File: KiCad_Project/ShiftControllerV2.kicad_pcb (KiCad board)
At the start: 2 copper layers, 102.9 x 43.2 mm, 25 parts, among them J1 SOLENOID, J2 PWR + I/O, Q1 BTN8982TA, Q2 BTN8982TA, U1 ControllerBoardV1

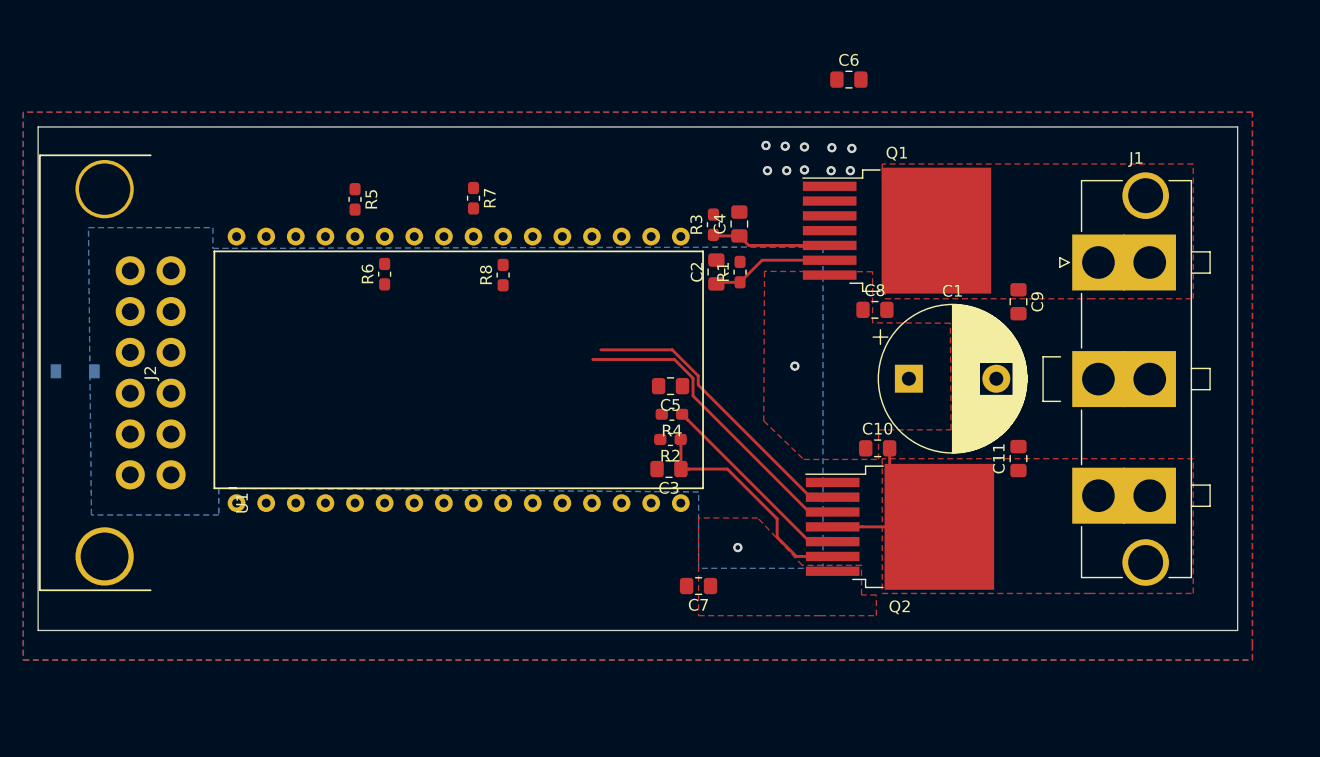
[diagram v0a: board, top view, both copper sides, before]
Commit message: Layout almost complete
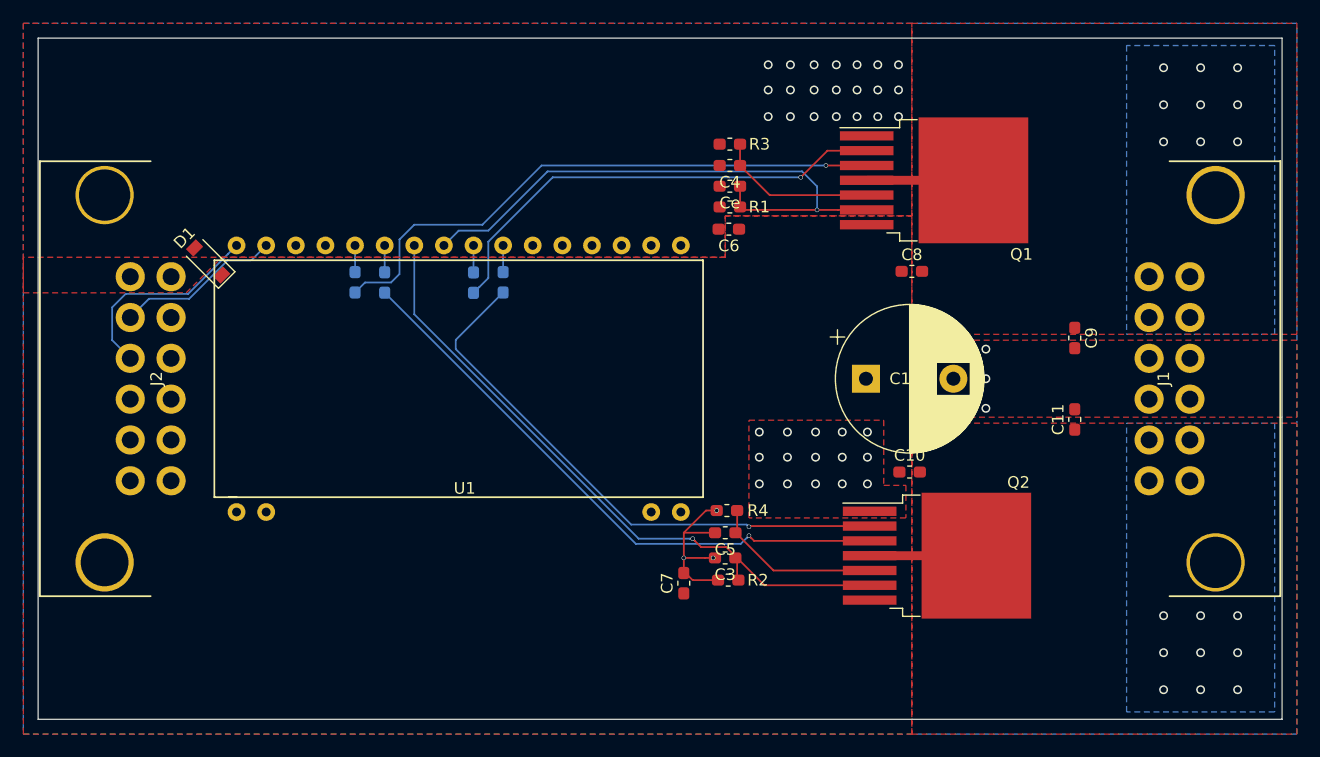
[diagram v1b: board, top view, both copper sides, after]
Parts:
- removed C2: 1n, Capacitor_SMD:C_0805_2012Metric_Pad1.15x1.40mm_HandSolder
- added Ce: 1n, Capacitor_SMD:C_0603_1608Metric_Pad1.05x0.95mm_HandSolder, F.Cu at (135.5, 81.3)
- C10, C11, C3, C4, C5, C6, C7, C8, C9: footprint Capacitor_SMD:C_0805_2012Metric_Pad1.15x1.40mm_HandSolder -> Capacitor_SMD:C_0603_1608Metric_Pad1.05x0.95mm_HandSolder
- D1: moved to F.Cu
- J1: value SOLENOID -> Conn_02x06_Top_Bottom; footprint Connector_Molex:Molex_Mini-Fit_Sr_42819-32XX_1x03_P10.00mm_Vertical -> Lukas_Library:MX120G
- J2: value PWR + I/O -> Conn_02x06_Top_Bottom
- R5, R6, R7, R8: moved to B.Cu
- moved C6 16.4 mm to (135.4, 85.0), turned to 180 degrees
- moved D1 14.8 mm to (90.8, 87.7), turned to 135 degrees
- moved C5 13.4 mm to (135.1, 111.0)
- moved R2 13.0 mm to (135.4, 115.1)
- moved J1 11.7 mm to (173.2, 97.8), turned to 270 degrees
- moved R4 9.51 mm to (135.3, 109.1)
- moved C3 9.01 mm to (135.1, 113.2)
- moved R7 7.24 mm to (113.5, 89.5), turned to 90 degrees
- moved R5 7.11 mm to (103.4, 89.5), turned to 90 degrees
- moved R3 7.05 mm to (135.5, 77.7), turned to 180 degrees
- moved C11 5.88 mm to (165.1, 101.3)
- moved C9 5.74 mm to (165.1, 94.3)
- moved R1 5.66 mm to (135.5, 83.1), turned to 180 degrees
- moved Q1 5.36 mm to (153.0, 80.8)
- moved C4 5.08 mm to (135.5, 79.5), turned to 180 degrees
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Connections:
- J1 pad 1: OUT1 -> OUT2
- J1 pad 2: GND -> OUT2
- J1 pad 3: OUT2 -> GND
- J2 pad 1: +12V -> GND
- J2 pad 11: GND -> (no net)
- J2 pad 12: +12V -> GND
- J2 pad 2: GND -> +12V
- J2 pad 3: CANL -> +12V
- J2 pad 4: CANH -> +12V
- J2 pad 5: GND -> +12V
- J2 pad 6: +12V -> GND
- J2 pad 7: +12V -> GND
- J2 pad 8: GND -> CANH
- J2 pad 9: (no net) -> CANL
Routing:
- net INH1: track 1.90 -> 50.1 mm, vias 0 -> 1
- net CURRENT1: track 10.6 -> 49.9 mm, vias 0 -> 1
- net IN1: track 1.90 -> 40.6 mm, vias 0 -> 1
- net CURRENT2: track 19.6 -> 56.5 mm, vias 0 -> 1
- net INH2: track 26.9 -> 51.0 mm, vias 0 -> 1
- net IN2: track 25.6 -> 48.4 mm, vias 0 -> 1
- net CANL: track 0.00 -> 17.9 mm
- net GND: track 0.00 -> 15.2 mm, vias 10 -> 47
- net CANH: track 0.00 -> 14.2 mm
- net OUT1: track 0.00 -> 9.15 mm, vias 0 -> 9
- net OUT2: track 17.6 -> 9.15 mm, vias 0 -> 9
- net Net-(C4-Pad1): track 10.3 -> 13.7 mm
- net Net-(C5-Pad1): track 17.4 -> 14.7 mm
- net Net-(R7-Pad2): track 0.00 -> 2.31 mm
- net Net-(R6-Pad2): track 0.00 -> 2.30 mm
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- added copper zone on B.Cu, net OUT1
- added copper zone on B.Cu, net OUT2
- removed copper zone on B.Cu, net +12V
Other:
- board size 102.9 x 43.2 mm -> 106.7 x 58.4 mm
- net class Default: clearance 0.2 -> 0.1524; trace_width 0.25 -> 0.1524; via_dia 0.8 -> 0.381; via_drill 0.4 -> 0.3048
- net class Power added: clearance 0.254, trace_width 0.762, via_dia 0.635, via_drill 0.381
- rule trace_clearance: 0.2 -> 0.1524
- rule trace_min: 0.2 -> 0.1524
- rule via_min_drill: 0.3 -> 0.2794
- rule via_min_size: 0.4 -> 0.381
